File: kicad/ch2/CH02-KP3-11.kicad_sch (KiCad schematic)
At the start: 7 parts

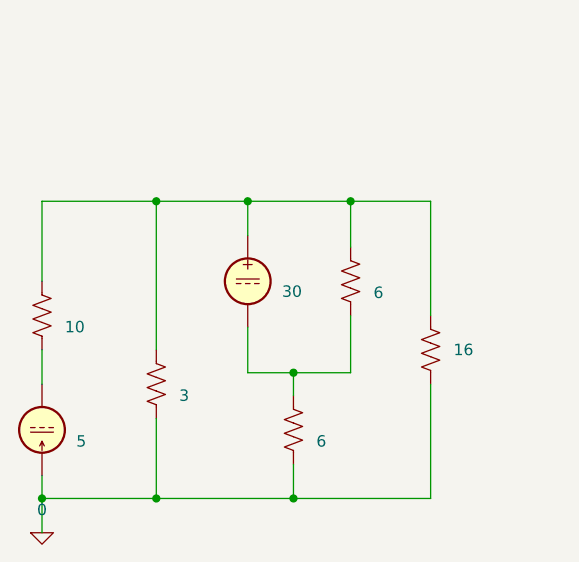
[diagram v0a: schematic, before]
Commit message: regular
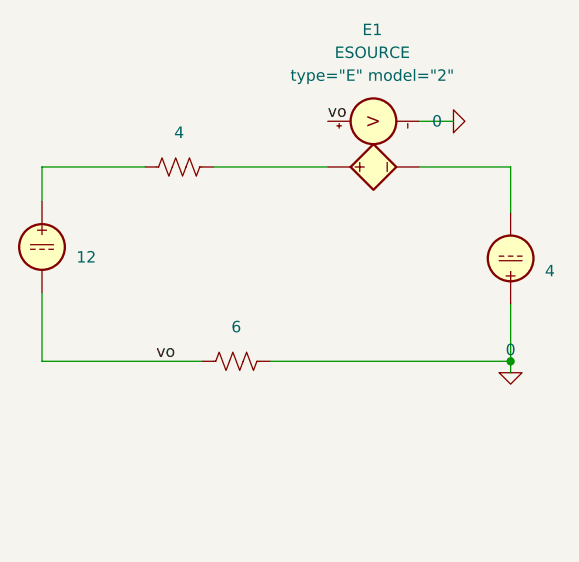
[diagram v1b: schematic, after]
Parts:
- removed I6: 5, symbol Simulation_SPICE:IDC
- removed R29: 10, symbol Device:R_US
- removed R30: 3, symbol Device:R_US
- removed R31, R32: 6, symbol Device:R_US
- removed R33: 16, symbol Device:R_US
- removed V12: 30, symbol Simulation_SPICE:VDC
- added E1: ESOURCE, symbol Simulation_SPICE:ESOURCE
- added R37: 4, symbol Device:R_US
- added R38: 6, symbol Device:R_US
- added V13: 12, symbol Simulation_SPICE:VDC
- added V14: 4, symbol Simulation_SPICE:VDC
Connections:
- net 0: now also E1.4 (C-), R38.2, V14.1
- new net: R37.1, V13.1
- new net: E1.1 (N+), R37.2
- new net: E1.2 (N-), V14.2
- new net vo: E1.3 (C+), R38.1, V13.2
